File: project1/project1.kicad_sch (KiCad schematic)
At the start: 21 parts, among them U2 MCP2515-xST, U3 STM32G474RBTx, U4 SN65HVD230, Y1 8MHz

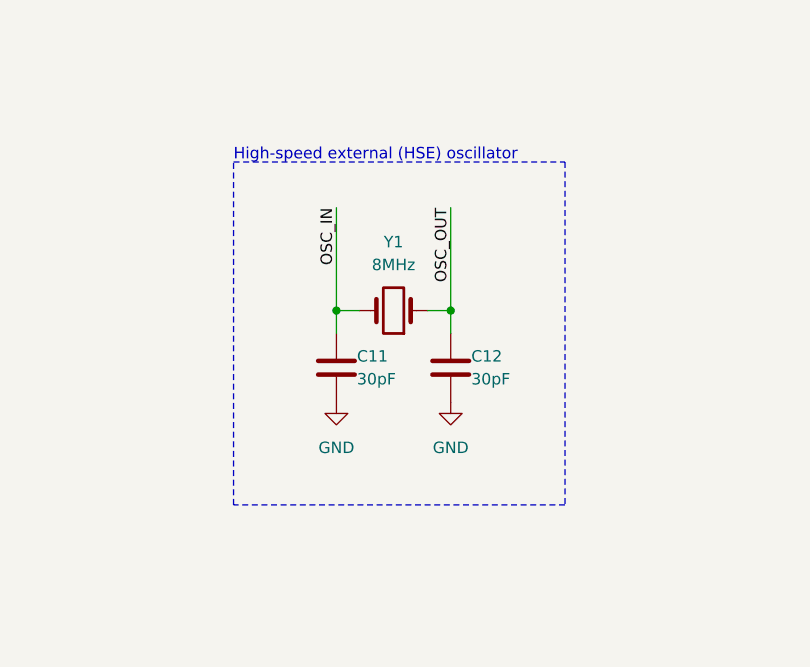
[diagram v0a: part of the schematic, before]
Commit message: qqchose a été fait
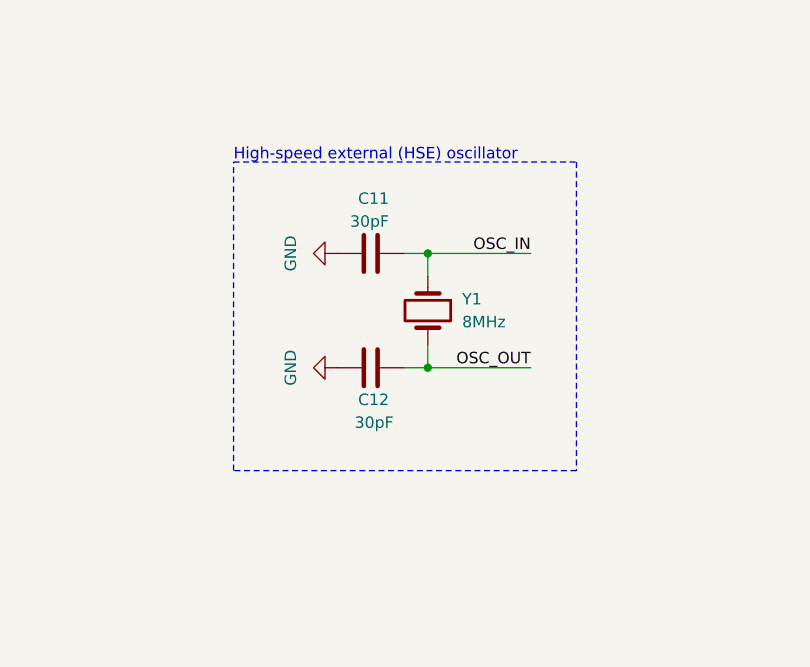
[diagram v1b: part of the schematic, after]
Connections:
- net GND: now also C11.1, C12.1; no longer C11.2, C12.2
- net OSC_IN: now also C11.2, Y1.1; no longer C11.1, Y1.2
- net OSC_OUT: now also C12.2, Y1.2; no longer C12.1, Y1.1
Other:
- moved on the sheet: C11, C12, Y1
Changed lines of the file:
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@@
 	)
 	(junction
-		(at 118.11 66.04)
+		(at 128.27 59.69)
 		(diameter 0)
 		(color 0 0 0 0)
@@
 	)
 	(junction
-		(at 130.81 66.04)
+		(at 128.27 72.39)
 		(diameter 0)
 		(color 0 0 0 0)
@@
 	(wire
 		(pts
-			(xy 118.11 54.61) (xy 118.11 66.04)
-		)
-		(stroke
-			(width 0)
-			(type default)
-		)
-	)
-	(wire
-		(pts
-			(xy 118.11 68.58) (xy 118.11 66.04)
+			(xy 139.7 59.69) (xy 128.27 59.69)
+		)
+		(stroke
+			(width 0)
+			(type default)
+		)
+	)
+	(wire
+		(pts
+			(xy 125.73 59.69) (xy 128.27 59.69)
 		)
 		(stroke
@@
 	(wire
 		(pts
-			(xy 118.11 66.04) (xy 120.65 66.04)
+			(xy 128.27 59.69) (xy 128.27 62.23)
 		)
 		(stroke
@@
 	(wire
 		(pts
-			(xy 130.81 54.61) (xy 130.81 66.04)
+			(xy 139.7 72.39) (xy 128.27 72.39)
 		)
 		(stroke
@@
 	(wire
 		(pts
-			(xy 130.81 66.04) (xy 128.27 66.04)
+			(xy 128.27 72.39) (xy 128.27 69.85)
 		)
 		(stroke
@@
 	(wire
 		(pts
-			(xy 130.81 68.58) (xy 130.81 66.04)
+			(xy 125.73 72.39) (xy 128.27 72.39)
 		)
 		(stroke
@@
 	(rectangle
 		(start 106.68 49.53)
-		(end 143.51 87.63)
+		(end 144.78 83.82)
 		(stroke
 			(width 0)
@@
 	)
 	(label "OSC_OUT"
-		(at 130.81 54.61 270)
+		(at 139.7 72.39 180)
 		(fields_autoplaced yes)
 		(effects
@@
 	)
 	(label "OSC_IN"
-		(at 118.11 54.61 270)
+		(at 139.7 59.69 180)
 		(fields_autoplaced yes)
 		(effects
@@
 	(symbol
 		(lib_id "Device:C")
-		(at 130.81 72.39 0)
+		(at 121.92 72.39 90)
 		(unit 1)
 		(exclude_from_sim no)
@@
 		(dnp no)
 		(property "Reference" "C12"
-			(at 133.096 71.12 0)
+			(at 123.952 75.946 90)
 			(effects
 				(font
@@
 		)
 		(property "Value" "30pF"
-			(at 133.096 73.66 0)
+			(at 124.46 78.486 90)
 			(effects
 				(font
@@
 		)
 		(property "Footprint" ""
-			(at 131.7752 76.2 0)
+			(at 125.73 71.4248 0)
 			(effects
 				(font
@@
 		)
 		(property "Datasheet" "~"
-			(at 130.81 72.39 0)
+			(at 121.92 72.39 0)
 			(effects
 				(font
@@
 		)
 		(property "Description" "Unpolarized capacitor"
-			(at 130.81 72.39 0)
+			(at 121.92 72.39 0)
 			(effects
 				(font
@@
 	(symbol
 		(lib_id "Device:C")
-		(at 118.11 72.39 0)
+		(at 121.92 59.69 90)
 		(unit 1)
 		(exclude_from_sim no)
@@
 		(dnp no)
 		(property "Reference" "C11"
-			(at 120.396 71.12 0)
+			(at 123.952 53.594 90)
 			(effects
 				(font
@@
 		)
 		(property "Value" "30pF"
-			(at 120.396 73.66 0)
+			(at 123.952 56.134 90)
 			(effects
 				(font
@@
 		)
 		(property "Footprint" ""
-			(at 119.0752 76.2 0)
+			(at 125.73 58.7248 0)
 			(effects
 				(font
@@
 		)
 		(property "Datasheet" "~"
-			(at 118.11 72.39 0)
+			(at 121.92 59.69 0)
 			(effects
 				(font
@@
 		)
 		(property "Description" "Unpolarized capacitor"
-			(at 118.11 72.39 0)
+			(at 121.92 59.69 0)
 			(effects
 				(font
@@
 	(symbol
 		(lib_id "power:GND")
-		(at 130.81 76.2 0)
+		(at 118.11 72.39 270)
 		(unit 1)
 		(exclude_from_sim no)
@@
 		(fields_autoplaced yes)
 		(property "Reference" "#PWR012"
-			(at 130.81 82.55 0)
+			(at 111.76 72.39 0)
 			(effects
 				(font
@@
 		)
 		(property "Value" "GND"
-			(at 130.81 81.28 0)
+			(at 113.03 72.39 0)
 			(effects
 				(font
@@
 		)
 		(property "Footprint" ""
-			(at 130.81 76.2 0)
+			(at 118.11 72.39 0)
 			(effects
 				(font
@@
 		)
 		(property "Datasheet" ""
-			(at 130.81 76.2 0)
+			(at 118.11 72.39 0)
 			(effects
 				(font
@@
 		)
 		(property "Description" "Power symbol creates a global label with name \"GND\" , ground"
-			(at 130.81 76.2 0)
+			(at 118.11 72.39 0)
 			(effects
 				(font
@@
 	(symbol
 		(lib_id "Exo_Symbol_Library:External_Oscillator")
-		(at 124.46 66.04 180)
+		(at 128.27 66.04 270)
 		(unit 1)
 		(exclude_from_sim no)
@@
 		(fields_autoplaced yes)
 		(property "Reference" "Y1"
-			(at 124.46 58.42 0)
-			(effects
-				(font
-					(size 1.27 1.27)
-				)
+			(at 132.08 64.7699 90)
+			(effects
+				(font
+					(size 1.27 1.27)
+				)
+				(justify left)
 			)
 		)
 		(property "Value" "8MHz"
-			(at 124.46 60.96 0)
-			(effects
-				(font
-					(size 1.27 1.27)
-				)
+			(at 132.08 67.3099 90)
+			(effects
+				(font
+					(size 1.27 1.27)
+				)
+				(justify left)
 			)
 		)
 		(property "Footprint" "Exocet:Crystal_SMD_HC49-SD"
-			(at 124.46 66.04 0)
+			(at 128.27 66.04 0)
 			(effects
 				(font
@@
 		)
 		(property "Datasheet" "~"
-			(at 124.46 66.04 0)
+			(at 128.27 66.04 0)
 			(effects
 				(font
@@
 		)
 		(property "Description" "Two pin crystal"
-			(at 124.46 66.04 0)
+			(at 128.27 66.04 0)
 			(effects
 				(font
@@
 		)
 		(property "JLCPCB" "C12674"
-			(at 124.46 66.04 0)
+			(at 128.27 66.04 0)
 			(effects
 				(font
@@
 		)
 		(property "Part Name" "X49SM8MSD2SC"
-			(at 124.46 66.04 0)
+			(at 128.27 66.04 0)
 			(effects
 				(font
@@
 	(symbol
 		(lib_id "power:GND")
-		(at 118.11 76.2 0)
+		(at 118.11 59.69 270)
 		(unit 1)
 		(exclude_from_sim no)
@@
 		(fields_autoplaced yes)
 		(property "Reference" "#PWR011"
-			(at 118.11 82.55 0)
+			(at 111.76 59.69 0)
 			(effects
 				(font
@@
 		)
 		(property "Value" "GND"
-			(at 118.11 81.28 0)
+			(at 113.03 59.69 0)
 			(effects
 				(font
@@
 		)
 		(property "Footprint" ""
-			(at 118.11 76.2 0)
+			(at 118.11 59.69 0)
 			(effects
 				(font
@@
 		)
 		(property "Datasheet" ""
-			(at 118.11 76.2 0)
+			(at 118.11 59.69 0)
 			(effects
 				(font
@@
 		)
 		(property "Description" "Power symbol creates a global label with name \"GND\" , ground"
-			(at 118.11 76.2 0)
-			(effects
-				(font
+			(at 118.11 59.69 0)
+			(effects
+				(font
